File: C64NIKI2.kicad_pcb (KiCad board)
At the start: 2 copper layers, 25 parts, among them J1 C64-EXP, Q1 BC237, SW1 FREEZE, SW2 RESET, U1 74LS74, U2 74LS163, U3 74LS125, U4 74LS05, U5 74LS174, U6 27C256

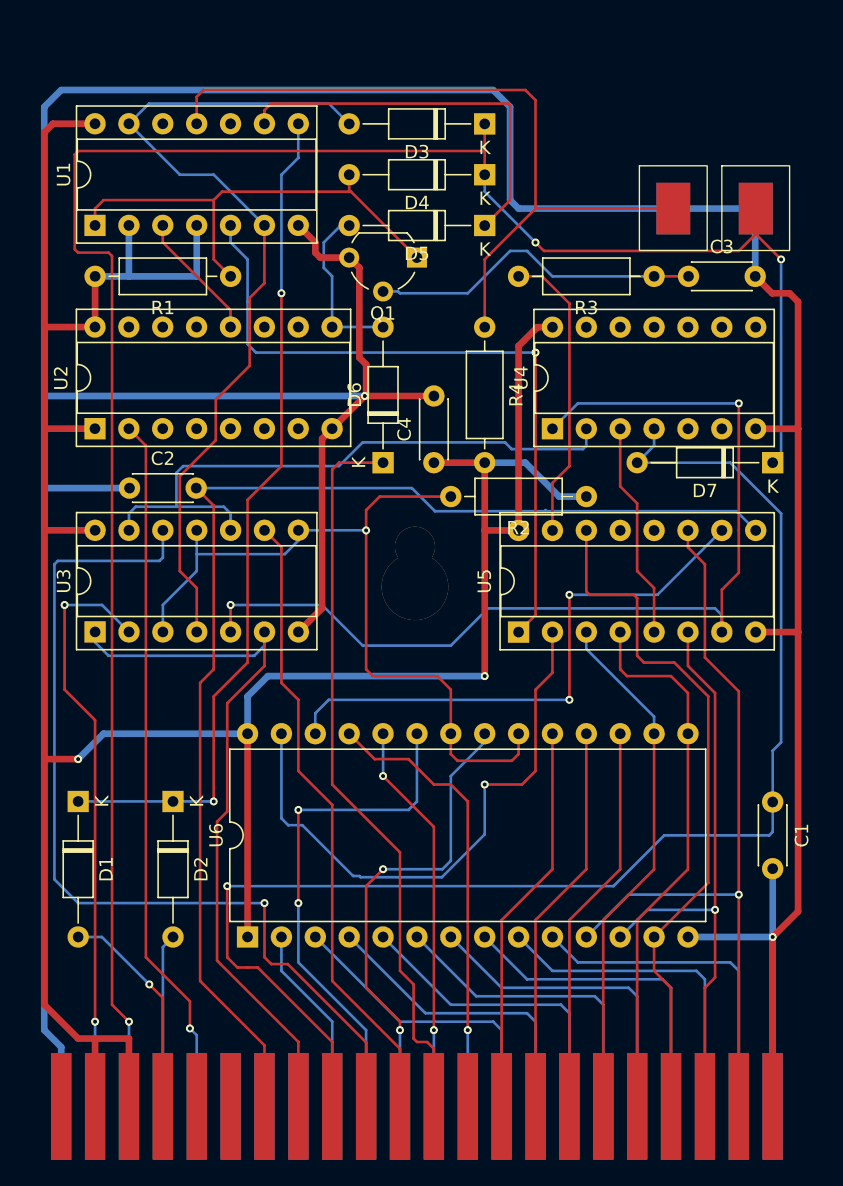
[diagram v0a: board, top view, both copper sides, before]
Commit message: first release
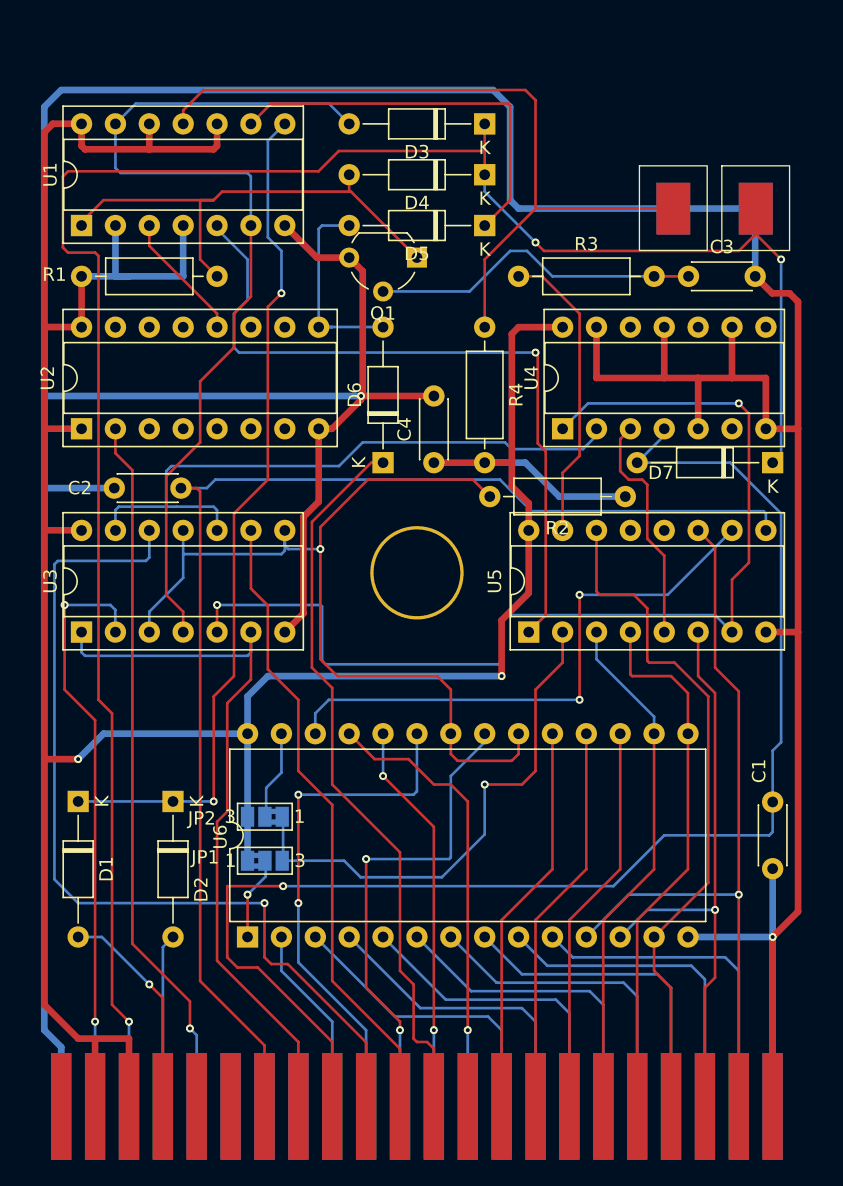
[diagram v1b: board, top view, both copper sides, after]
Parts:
- added JP1: 1-2 = 27C - 2-3 = 28C, C64NIKI2:BottomSolderJumper-3_P1.3mm_Bridged2Bar12_Pad1.0x1.5mm_NumberLabels, F.Cu at (109.2, 154.3)
- added JP2: 1-2 = 27C - 2-3 = 28C, C64NIKI2:BottomSolderJumper-3_P1.3mm_Bridged2Bar12_Pad1.0x1.5mm_NumberLabels, F.Cu at (109.2, 151.0)
- moved R2 2.92 mm to (136.3, 127.0)
- moved C2 1.14 mm to (98.0, 126.4)
- moved U3 1.02 mm to (95.5, 137.2)
- moved R1 1.02 mm to (105.7, 110.5)
- moved U1 1.01 mm to (95.5, 106.7)
- moved U2 1.01 mm to (95.5, 121.9)
- moved U4 0.76 mm to (131.6, 121.9)
- moved U5 0.76 mm to (129.0, 137.2)
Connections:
- net /EXP_10 renamed /IO2
- net /EXP_11 renamed /ROML
- net /EXP_4 renamed /IRQ
- net /EXP_5 renamed /RW
- net /EXP_7 renamed /IO1
- net /EXP_8 renamed /GAME
- net /EXP_9 renamed /EXROM
- net /EXP_B renamed /ROMH
- net /EXP_C renamed /RESET
- net /EXP_D renamed /NMI
- net /EXP_E renamed /PHI2
- U4 pad 11: unconnected-(U4-Pad11) -> GND
- U4 pad 13: unconnected-(U4-Pad13) -> GND
- U4 pad 5: unconnected-(U4-Pad5) -> GND
- U4 pad 9: unconnected-(U4-Pad9) -> GND
- U5 pad 2: Net-(U5-Q0) -> Net-(JP1-B)
- U6 pad 1: VCC -> Net-(JP1-C)
- U6 pad 27: Net-(U5-Q0) -> Net-(JP2-C)
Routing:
- net Net-(U5-Q0): track 43.7 -> 0.00 mm, vias 1 -> 0
- net Net-(JP1-B): track 0.00 -> 39.5 mm, vias 0 -> 1
- net GND: track 309.5 -> 339.9 mm
- net Net-(U6-~{CE}): track 60.1 -> 69.0 mm
- net VCC: track 218.0 -> 226.6 mm
- net Net-(JP2-C): track 0.00 -> 6.70 mm
- net Net-(JP1-C): track 0.00 -> 6.28 mm, vias 0 -> 1
- net Net-(U5-Q2): track 75.2 -> 80.7 mm
- net Net-(D3-A): track 64.7 -> 69.8 mm
- net /IO1: track 92.7 -> 96.1 mm
- net Net-(D5-A): track 12.9 -> 15.6 mm
- net Net-(U1A-Q): track 52.8 -> 55.1 mm
- net Net-(U3-Pad10): track 46.4 -> 47.8 mm
- net Net-(D4-A): track 35.5 -> 36.9 mm
- net Net-(U5-Q1): track 16.3 -> 17.5 mm
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
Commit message: First printed revision
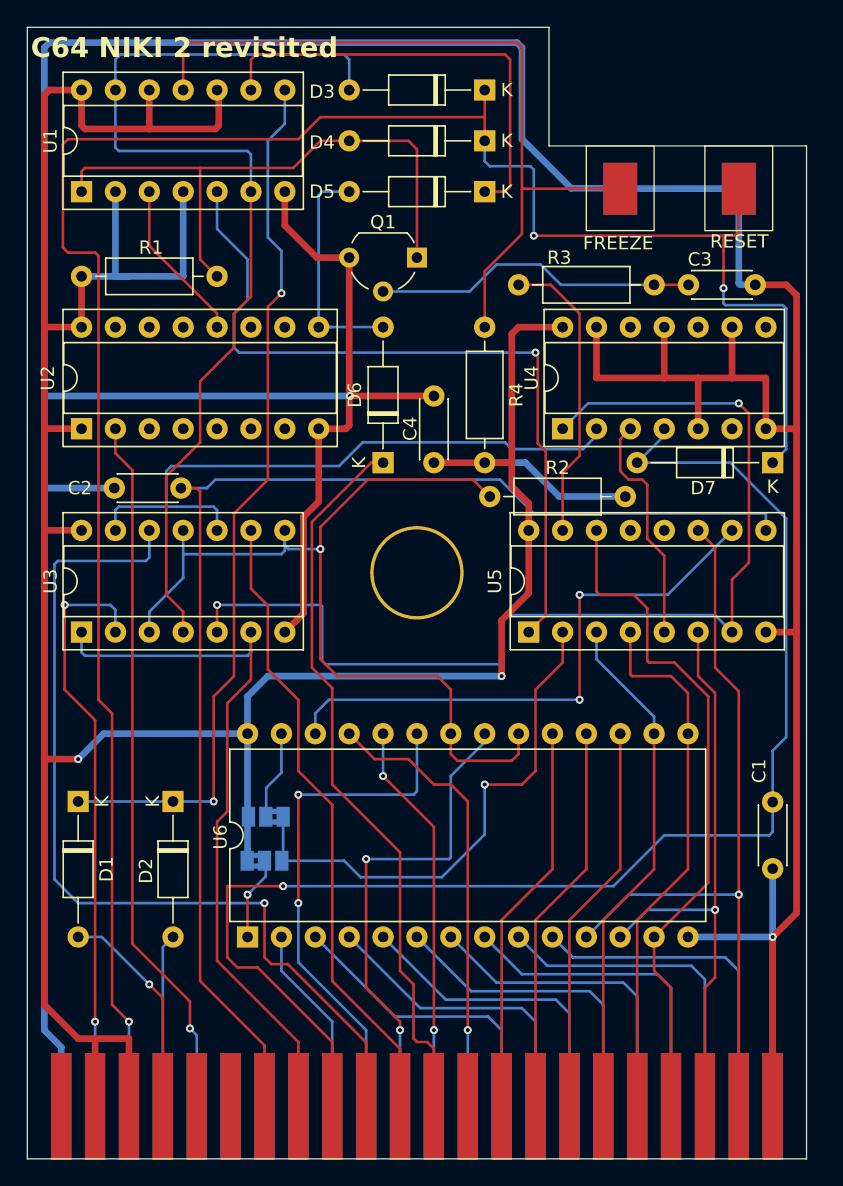
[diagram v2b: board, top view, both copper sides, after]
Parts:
- moved SW1 4.25 mm to (134.6, 105.8)
- moved D3 2.54 mm to (125.7, 96.5)
- moved D4 2.54 mm to (125.7, 100.3)
- moved D5 2.54 mm to (125.7, 104.1)
- moved U1 2.54 mm to (95.5, 104.1)
- moved SW2 1.96 mm to (143.5, 105.8)
- moved C3 0.64 mm to (141.0, 111.1)
- moved R3 0.64 mm to (138.4, 111.1)
- moved JP2 0.07 mm to (109.3, 151.0)
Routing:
- net VCC: track 226.6 -> 237.6 mm
- net /RESET: track 153.2 -> 162.7 mm
- net GND: track 339.9 -> 348.8 mm
- net Net-(D4-A): track 36.9 -> 44.7 mm
- net Net-(D3-A): track 69.8 -> 76.1 mm
- net Net-(D5-K): track 29.9 -> 33.6 mm
- net Net-(U1A-Q): track 55.1 -> 58.5 mm
- net Net-(U1A-C): track 9.72 -> 12.3 mm
- net Net-(D1-K): track 64.0 -> 66.6 mm
- net Net-(D5-A): track 15.6 -> 18.1 mm
- net Net-(U1B-C): track 57.3 -> 58.4 mm
- net Net-(Q1-B): track 24.9 -> 24.4 mm
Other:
- board outline added: 58.4 x 84.8 mm
- board text added: "C64 NIKI 2 revisited"
- board text added: "FREEZE"
- board text added: "RESET"
